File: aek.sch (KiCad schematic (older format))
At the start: 225 parts, among them J1 Conn_01x04_MountingPin, SW1 SW_Push, U1 ATmega32U4-AU, Y1 16MHz

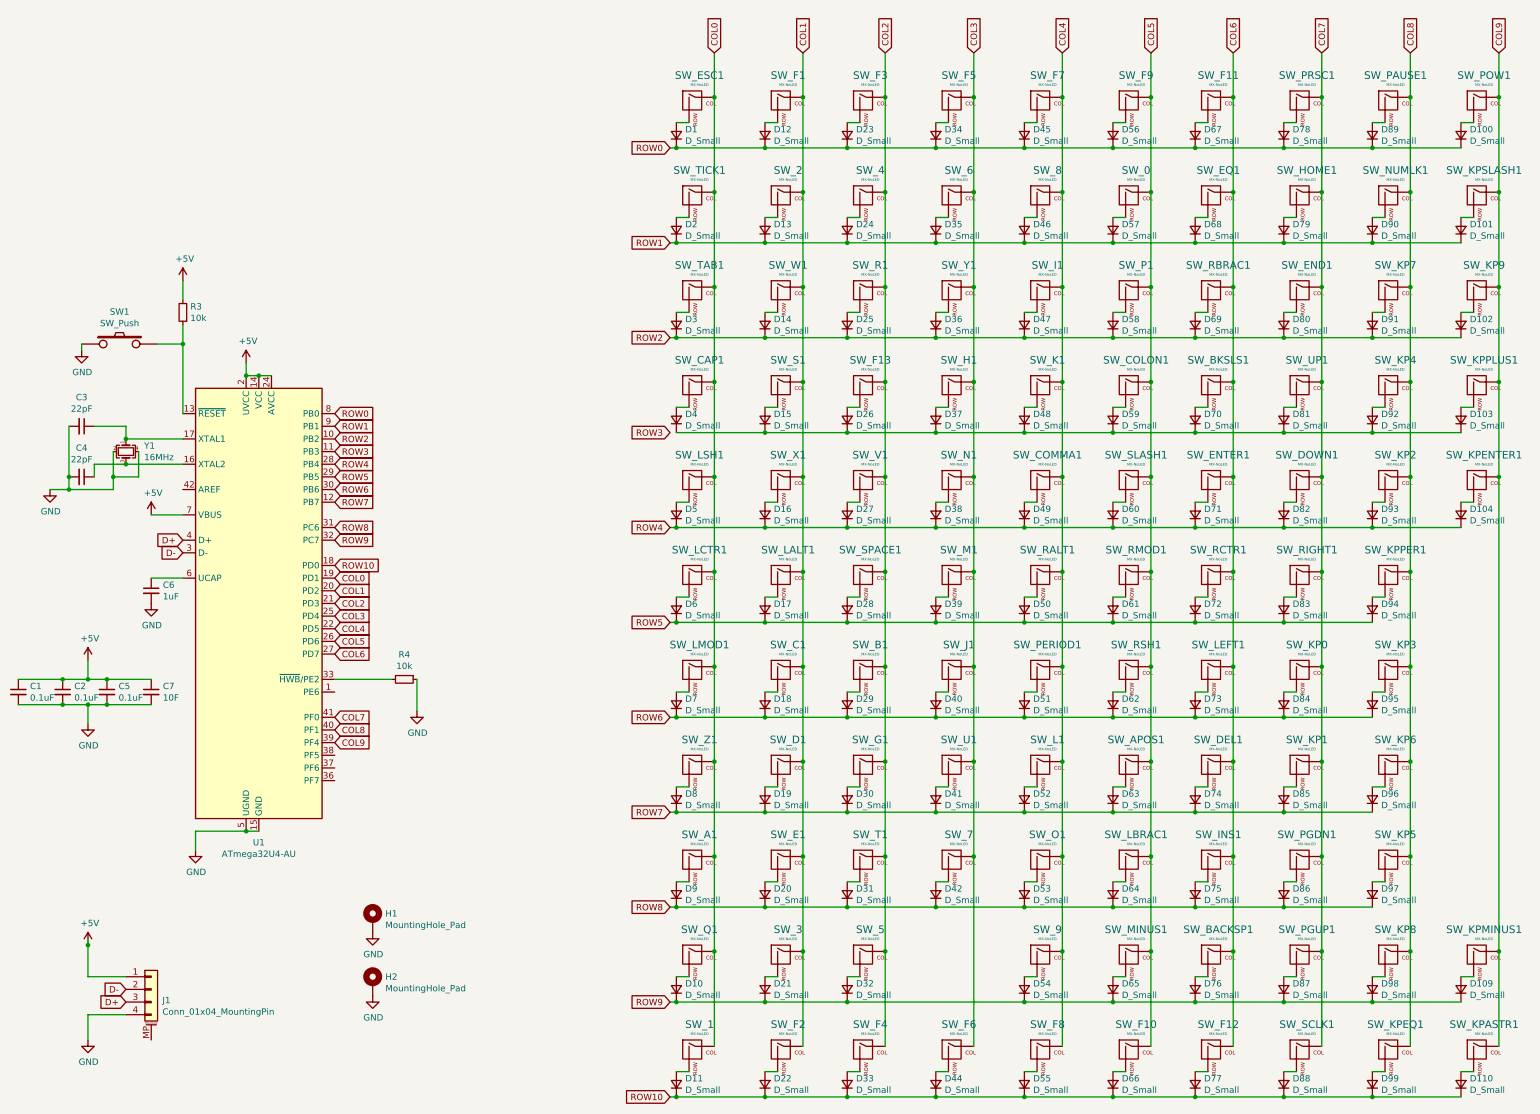
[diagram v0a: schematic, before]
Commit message: first draft
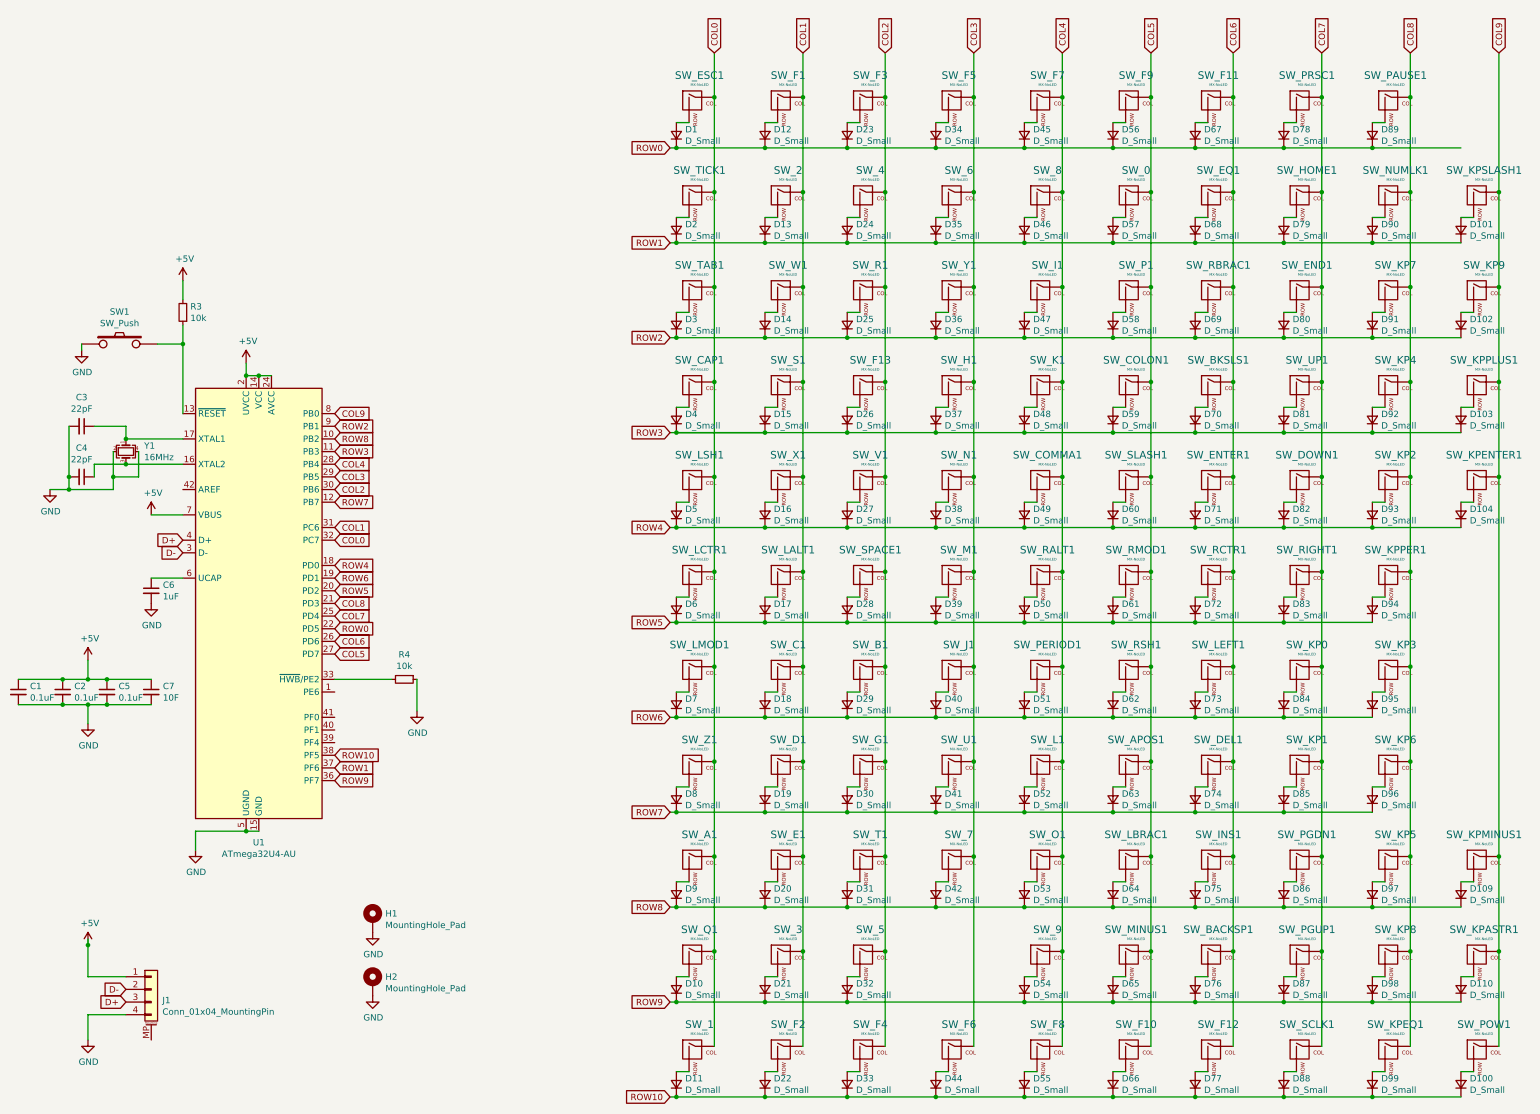
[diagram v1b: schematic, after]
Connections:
- net COL0: now also U1.32 (PC7); no longer U1.19 (PD1)
- net COL1: now also U1.31 (PC6); no longer U1.20 (PD2)
- net COL2: now also U1.30 (PB6); no longer U1.21 (PD3)
- net COL3: now also U1.29 (PB5); no longer U1.25 (PD4)
- net COL4: now also U1.28 (PB4); no longer U1.22 (PD5)
- net COL5: now also U1.27 (PD7); no longer U1.26 (PD6)
- net COL6: now also U1.26 (PD6); no longer U1.27 (PD7)
- net COL7: now also U1.25 (PD4); no longer U1.41 (PF0)
- net COL8: now also U1.21 (PD3); no longer U1.40 (PF1)
- net COL9: now also U1.8 (PB0); no longer U1.39 (PF4)
- net ROW0: now also U1.22 (PD5); no longer D100.1 (K), U1.8 (PB0)
- net ROW1: now also U1.37 (PF6); no longer U1.9 (PB1)
- net ROW10: now also D100.1 (K), U1.38 (PF5); no longer D110.1 (K), U1.18 (PD0)
- net ROW2: now also U1.9 (PB1); no longer U1.10 (PB2)
- net ROW3: now also D103.1 (K), D15.1 (K), D26.1 (K), D37.1 (K), D4.1 (K), D48.1 (K), D59.1 (K), D70.1 (K), D81.1 (K), D92.1 (K)
- net ROW4: now also U1.18 (PD0); no longer U1.28 (PB4)
- net ROW5: now also U1.20 (PD2); no longer U1.29 (PB5)
- net ROW6: now also U1.19 (PD1); no longer U1.30 (PB6)
- net ROW8: now also D109.1 (K), U1.10 (PB2); no longer U1.31 (PC6)
- net ROW9: now also D110.1 (K), U1.36 (PF7); no longer D109.1 (K), U1.32 (PC7)
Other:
- moved on the sheet: D100, D109, D110, SW_KPASTR1, SW_KPMINUS1, SW_POW1
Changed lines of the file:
@@
 Wire Wire Line
 	8200 7500 8200 9000
-Connection ~ 12350 1500
 Connection ~ 11650 1500
 Connection ~ 10950 1500
@@
 Connection ~ 6850 1500
 Wire Wire Line
-	12350 1500 12350 1150
-Wire Wire Line
-	12350 1500 12350 2250
-Wire Wire Line
 	11650 1500 11650 1150
 Wire Wire Line
@@
 ROW0
 Wire Wire Line
-	12050 9200 12150 9200
+	12050 8450 12150 8450
 $Comp
 L Device:D_Small D110
 U 1 1 6145A318
-P 12050 9300
-F 0 "D110" V 12096 9230 50  0000 R CNN
-F 1 "D_Small" V 12005 9230 50  0000 R CNN
-F 2 "Diode_SMD:D_SOD-123" V 12050 9300 50  0001 C CNN
-F 3 "~" V 12050 9300 50  0001 C CNN
-	1    12050 9300
+P 12050 8550
+F 0 "D110" V 12096 8480 50  0000 R CNN
+F 1 "D_Small" V 12005 8480 50  0000 R CNN
+F 2 "Diode_SMD:D_SOD-123" V 12050 8550 50  0001 C CNN
+F 3 "~" V 12050 8550 50  0001 C CNN
+	1    12050 8550
 	0    -1   -1   0
 $EndComp
@@
 Wire Wire Line
 	10650 9400 11350 9400
-Connection ~ 11350 9400
 Wire Wire Line
-	11350 9400 12050 9400
+	11350 8650 12050 8650
 Connection ~ 8600 9400
 Connection ~ 7200 9400
@@
 Wire Wire Line
 	11650 9000 11650 8250
-Wire Wire Line
-	12350 8250 12350 9000
 Connection ~ 6150 8250
 Connection ~ 6850 8250
@@
 Connection ~ 10950 8250
 Connection ~ 11650 8250
-Connection ~ 12350 8250
-Wire Wire Line
-	11350 1900 12050 1900
 Wire Wire Line
 	11350 2650 12050 2650
@@
 	11350 4900 12050 4900
 Wire Wire Line
-	11350 8650 12050 8650
-Connection ~ 11350 8650
+	11350 7900 12050 7900
 Connection ~ 11350 4900
 Connection ~ 11350 4150
 Connection ~ 11350 3400
 Connection ~ 11350 2650
-Connection ~ 11350 1900
 Wire Wire Line
 	6850 2250 6850 3000
@@
 L Device:D_Small D109
 U 1 1 6145A285
-P 12050 8550
-F 0 "D109" V 12096 8480 50  0000 R CNN
-F 1 "D_Small" V 12005 8480 50  0000 R CNN
-F 2 "Diode_SMD:D_SOD-123" V 12050 8550 50  0001 C CNN
-F 3 "~" V 12050 8550 50  0001 C CNN
-	1    12050 8550
+P 12050 7800
+F 0 "D109" V 12096 7730 50  0000 R CNN
+F 1 "D_Small" V 12005 7730 50  0000 R CNN
+F 2 "Diode_SMD:D_SOD-123" V 12050 7800 50  0001 C CNN
+F 3 "~" V 12050 7800 50  0001 C CNN
+	1    12050 7800
 	0    -1   -1   0
 $EndComp
 Wire Wire Line
-	12050 8450 12150 8450
+	12050 7700 12150 7700
 Wire Wire Line
 	7900 7700 8000 7700
@@
 Wire Wire Line
 	11350 1700 11450 1700
-$Comp
-L MX_Alps_Hybrid:MX-NoLED SW_POW1
-U 1 1 6126A487
-P 12200 1550
-F 0 "SW_POW1" H 12233 1773 60  0000 C CNN
-F 1 "MX-NoLED" H 12233 1699 20  0000 C CNN
-F 2 "MX_Alps_Hybrid:MX-1U-NoLED" H 11575 1525 60  0001 C CNN
-F 3 "" H 11575 1525 60  0001 C CNN
-	1    12200 1550
-	1    0    0    -1
-$EndComp
-$Comp
-L Device:D_Small D100
-U 1 1 6126A48D
-P 12050 1800
-F 0 "D100" V 12096 1730 50  0000 R CNN
-F 1 "D_Small" V 12005 1730 50  0000 R CNN
-F 2 "Diode_SMD:D_SOD-123" V 12050 1800 50  0001 C CNN
-F 3 "~" V 12050 1800 50  0001 C CNN
-	1    12050 1800
-	0    -1   -1   0
-$EndComp
-Wire Wire Line
-	12050 1700 12150 1700
 Wire Wire Line
 	1200 8750 1200 8950
@@
 L MX_Alps_Hybrid:MX-NoLED SW_KPASTR1
 U 1 1 6145A31E
-P 12200 9050
-F 0 "SW_KPASTR1" H 12233 9273 60  0000 C CNN
-F 1 "MX-NoLED" H 12233 9199 20  0000 C CNN
-F 2 "MX_Alps_Hybrid:MX-1U-NoLED" H 11575 9025 60  0001 C CNN
-F 3 "" H 11575 9025 60  0001 C CNN
-	1    12200 9050
+P 12200 8300
+F 0 "SW_KPASTR1" H 12233 8523 60  0000 C CNN
+F 1 "MX-NoLED" H 12233 8449 20  0000 C CNN
+F 2 "MX_Alps_Hybrid:MX-1U-NoLED" H 11575 8275 60  0001 C CNN
+F 3 "" H 11575 8275 60  0001 C CNN
+	1    12200 8300
 	1    0    0    -1
 $EndComp
 Wire Wire Line
-	12350 4500 12350 8250
+	12350 4500 12350 7500
 $Comp
 L MX_Alps_Hybrid:MX-NoLED SW_KPMINUS1
 U 1 1 6145A28B
-P 12200 8300
-F 0 "SW_KPMINUS1" H 12233 8523 60  0000 C CNN
-F 1 "MX-NoLED" H 12233 8449 20  0000 C CNN
-F 2 "MX_Alps_Hybrid:MX-1U-NoLED" H 11575 8275 60  0001 C CNN
-F 3 "" H 11575 8275 60  0001 C CNN
-	1    12200 8300
+P 12200 7550
+F 0 "SW_KPMINUS1" H 12233 7773 60  0000 C CNN
+F 1 "MX-NoLED" H 12233 7699 20  0000 C CNN
+F 2 "MX_Alps_Hybrid:MX-1U-NoLED" H 11575 7525 60  0001 C CNN
+F 3 "" H 11575 7525 60  0001 C CNN
+	1    12200 7550
 	1    0    0    -1
 $EndComp
@@
 	1    0    0    -1
 $EndComp
-Text GLabel 3150 4700 2    50   Input ~ 0
-ROW7
-Text GLabel 3150 4600 2    50   Input ~ 0
+Text GLabel 3150 5300 2    50   Input ~ 0
 ROW6
-Text GLabel 3150 4500 2    50   Input ~ 0
+Text GLabel 3150 5400 2    50   Input ~ 0
 ROW5
-Text GLabel 3150 4400 2    50   Input ~ 0
+Text GLabel 3150 5200 2    50   Input ~ 0
 ROW4
 Text GLabel 3150 4300 2    50   Input ~ 0
 ROW3
-Text GLabel 3150 4200 2    50   Input ~ 0
-ROW2
 Text GLabel 3150 4100 2    50   Input ~ 0
-ROW1
-Text GLabel 3150 4000 2    50   Input ~ 0
+ROW2
+Text GLabel 3150 5700 2    50   Input ~ 0
 ROW0
-Text GLabel 3150 4900 2    50   Input ~ 0
-ROW8
-Text GLabel 3150 5000 2    50   Input ~ 0
+Text GLabel 3150 6900 2    50   Input ~ 0
 ROW9
-Text GLabel 3150 5200 2    50   Input ~ 0
+Text GLabel 3150 6700 2    50   Input ~ 0
 ROW10
 Text GLabel 6150 1150 1    50   Input ~ 0
@@
 Text GLabel 12350 1150 1    50   Input ~ 0
 COL9
-Text GLabel 3150 6600 2    50   Input ~ 0
+Text GLabel 3150 4000 2    50   Input ~ 0
 COL9
-Text GLabel 3150 6500 2    50   Input ~ 0
+Text GLabel 3150 5500 2    50   Input ~ 0
 COL8
-Text GLabel 3150 6400 2    50   Input ~ 0
+Text GLabel 3150 5600 2    50   Input ~ 0
 COL7
-Text GLabel 3150 5900 2    50   Input ~ 0
-COL6
 Text GLabel 3150 5800 2    50   Input ~ 0
+COL6
+Text GLabel 3150 5900 2    50   Input ~ 0
 COL5
-Text GLabel 3150 5700 2    50   Input ~ 0
+Text GLabel 3150 4400 2    50   Input ~ 0
 COL4
-Text GLabel 3150 5600 2    50   Input ~ 0
+Text GLabel 3150 4500 2    50   Input ~ 0
 COL3
-Text GLabel 3150 5500 2    50   Input ~ 0
+Text GLabel 3150 4600 2    50   Input ~ 0
 COL2
-Text GLabel 3150 5400 2    50   Input ~ 0
+Text GLabel 3150 4900 2    50   Input ~ 0
 COL1
-Text GLabel 3150 5300 2    50   Input ~ 0
+Text GLabel 3150 5000 2    50   Input ~ 0
 COL0
 Wire Wire Line
@@
 	1    0    0    -1
 $EndComp
+Connection ~ 11350 1900
+Wire Wire Line
+	11350 1900 12050 1900
+Wire Wire Line
+	12350 1150 12350 2250
+Connection ~ 11350 7900
+Connection ~ 12350 7500
+Wire Wire Line
+	12350 7500 12350 8250
+Connection ~ 11350 8650
+Connection ~ 12350 8250
+Wire Wire Line
+	12350 8250 12350 9000
+$Comp
+L MX_Alps_Hybrid:MX-NoLED SW_POW1
+U 1 1 6126A487
+P 12200 9050
+F 0 "SW_POW1" H 12233 9273 60  0000 C CNN
+F 1 "MX-NoLED" H 12233 9199 20  0000 C CNN
+F 2 "MX_Alps_Hybrid:MX-1U-NoLED" H 11575 9025 60  0001 C CNN
+F 3 "" H 11575 9025 60  0001 C CNN
+	1    12200 9050
+	1    0    0    -1
+$EndComp
+$Comp
+L Device:D_Small D100
+U 1 1 6126A48D
+P 12050 9300
+F 0 "D100" V 12096 9230 50  0000 R CNN
+F 1 "D_Small" V 12005 9230 50  0000 R CNN
+F 2 "Diode_SMD:D_SOD-123" V 12050 9300 50  0001 C CNN
+F 3 "~" V 12050 9300 50  0001 C CNN
+	1    12050 9300
+	0    -1   -1   0
+$EndComp
+Wire Wire Line
+	12050 9200 12150 9200
+Wire Wire Line
+	12050 9400 11350 9400
+Connection ~ 11350 9400
+Wire Wire Line
+	5800 4150 5850 4150
+Connection ~ 5850 4150
+Wire Wire Line
+	5850 4150 6550 4150
+Text GLabel 3150 6800 2    50   Input ~ 0
+ROW1
+Text GLabel 3150 4200 2    50   Input ~ 0
+ROW8
+Text GLabel 3150 4700 2    50   Input ~ 0
+ROW7
 $EndSCHEMATC
